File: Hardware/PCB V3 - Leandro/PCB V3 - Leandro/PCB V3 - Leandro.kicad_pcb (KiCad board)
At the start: 2 copper layers, 70.2 x 30 mm, 13 parts, among them J1 Bateria (+), J10 MOTOR_DER, J3 Sensor TATAMI FD, J5 Sensor TATAMI FI, J6 STEP_DOWN, J7 IR_FD, J8 IR_FI, J9 MOTOR_IZQ, SW1 START, SW2 ESTRATEGIA, U1 ESP32_DevKit_V1_CH9102X

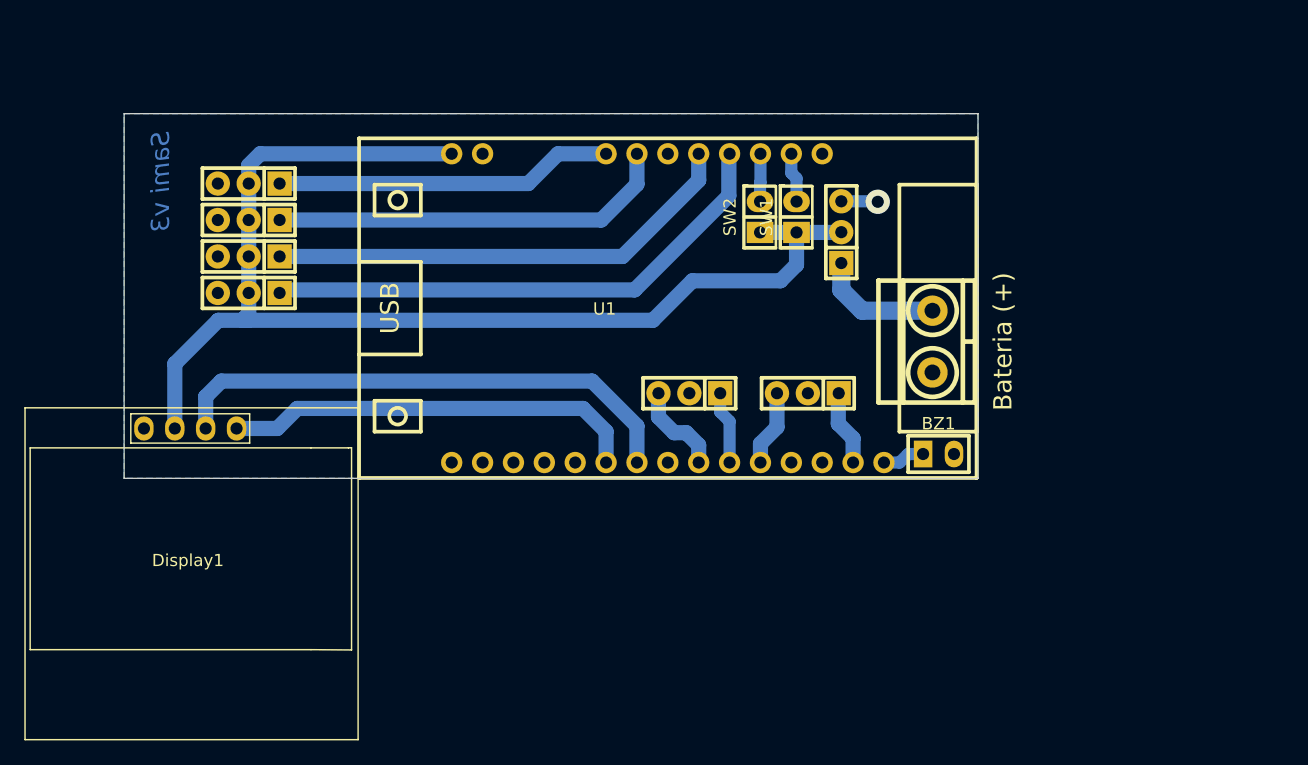
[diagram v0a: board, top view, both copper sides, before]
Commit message: placa para fabricar ya
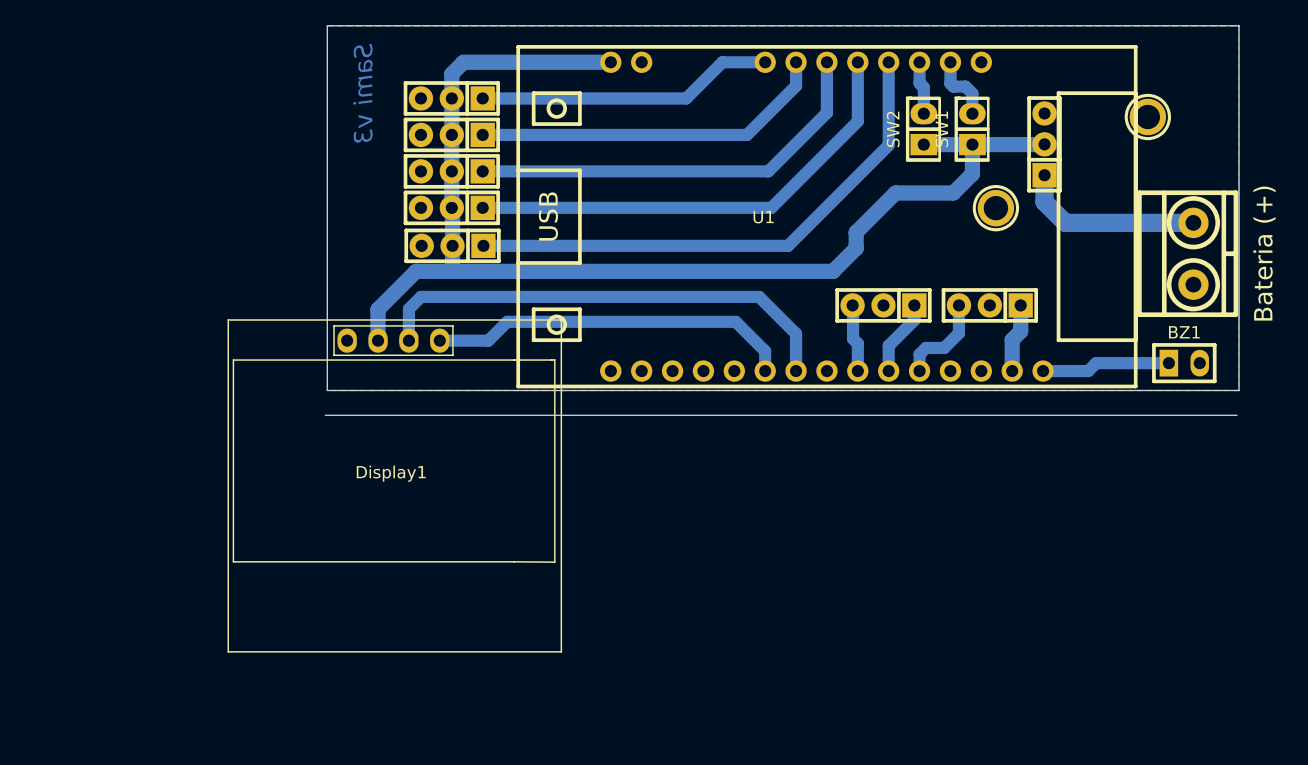
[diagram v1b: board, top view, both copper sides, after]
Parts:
- added H1: Mounting_Hole, EESTN5:pad_3mm, F.Cu at (174.2, 80.3)
- added H2: Mounting_Hole, EESTN5:pad_3mm, F.Cu at (161.7, 87.8)
- added J2: IR_COSTADO, EESTN5:Pin_Strip_3, F.Cu at (117.0, 90.9)
- moved J1 22.7 mm to (178.0, 91.5)
- moved BZ1 21.6 mm to (177.2, 100.5)
- moved Display1 18.2 mm to (112.0, 109.3)
- moved J6 18.2 mm to (165.7, 82.5)
- moved J3 18.1 mm to (117.0, 81.8)
- moved J5 18.1 mm to (117.0, 78.8)
- moved J7 18.1 mm to (117.0, 87.8)
- moved J8 18.1 mm to (117.0, 84.8)
- moved J9 17.5 mm to (152.5, 95.8)
- moved J10 16.6 mm to (161.2, 95.8)
- moved SW1 16.2 mm to (159.5, 81.3)
- moved SW2 15.3 mm to (155.5, 81.3)
- moved U1 15.1 mm to (149.1, 88.5)
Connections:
- U1 pad 6: /IR_FD -> /IR_COSTADO
- U1 pad 7: /IR_FI -> /IR_FD
- U1 pad 8: /IR_I -> /IR_FI
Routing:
- net /IR_COSTADO: track 0.00 -> 43.6 mm
- net /BUZZER: track 3.51 -> 10.6 mm
- net /IR_FD: track 43.7 -> 38.7 mm
- net /IR_FI: track 39.3 -> 34.5 mm
- net /Vstep: track 10.4 -> 15.2 mm
- net /SDA: track 34.4 -> 30.0 mm
- net /SCL: track 43.2 -> 39.2 mm
- net /TATAMI_FD: track 33.1 -> 29.4 mm
- net /TATAMI_FI: track 27.9 -> 24.5 mm
- net GND: track 3.75 -> 0.73 mm, vias 1 -> 0
- net /M2A: track 7.66 -> 5.58 mm
- net /M1A: track 6.26 -> 7.62 mm
- net /START: track 4.42 -> 5.56 mm
- net +5V: track 100.7 -> 99.7 mm
- net /M2B: track 6.10 -> 7.00 mm
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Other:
- board size 70.2 x 30 mm -> 75.2 x 32 mm
